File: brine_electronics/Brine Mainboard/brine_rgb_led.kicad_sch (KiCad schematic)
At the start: 3 parts

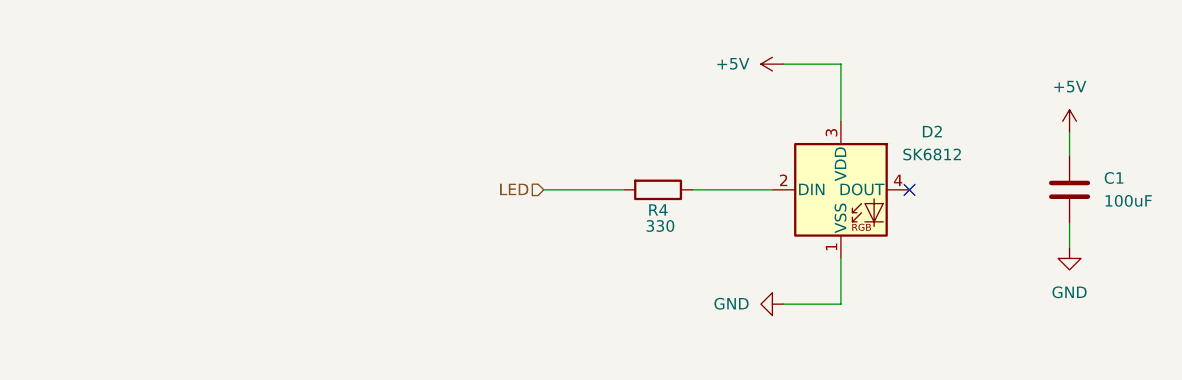
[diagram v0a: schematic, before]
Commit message: Updated PCB manufacturing files :mechanical_arm:
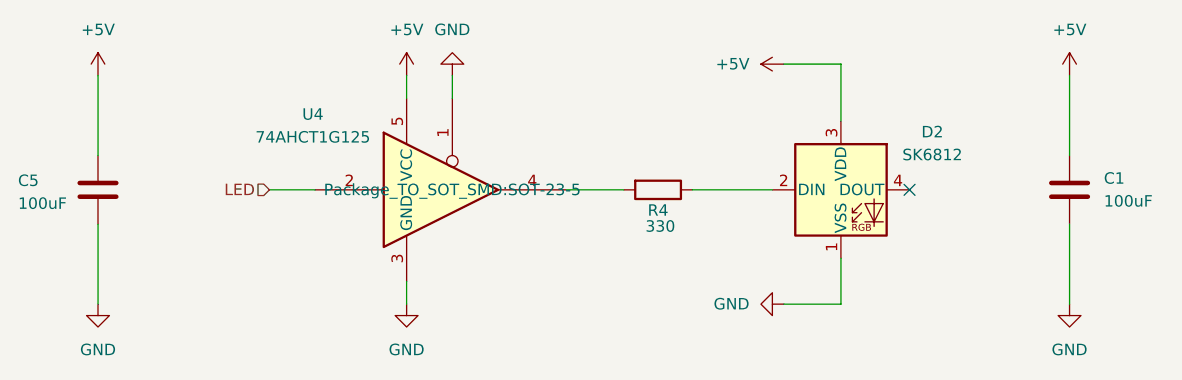
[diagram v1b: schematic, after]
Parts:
- added C5: 100uF, Capacitor_SMD:C_0805_2012Metric, symbol Device:C
- added U4: 74AHCT1G125, Package_TO_SOT_SMD:SOT-23-5, symbol 74xGxx:74AHCT1G125
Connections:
- net +5V: now also C5.1, U4.5 (VCC)
- net GND: now also C5.2, U4.1, U4.3 (GND)
- net LED: now also U4.2; no longer R4.2
- new net: R4.2, U4.4
